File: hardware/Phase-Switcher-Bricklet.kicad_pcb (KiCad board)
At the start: 2 copper layers, 70 x 46.4 mm, 43 parts, among them CN1 HC-GH-7PWTKK, P10 WJ124-3.81-4P, P20 WJ124-3.81-4P, P40 WJ124-3.81-2P, U1 XMC1302-Q024X0032-AB, U10 AQH2223, U11 6N139M, U20 AQH2223, U21 6N139M, U30 AQH2223, U40 AQY282SX

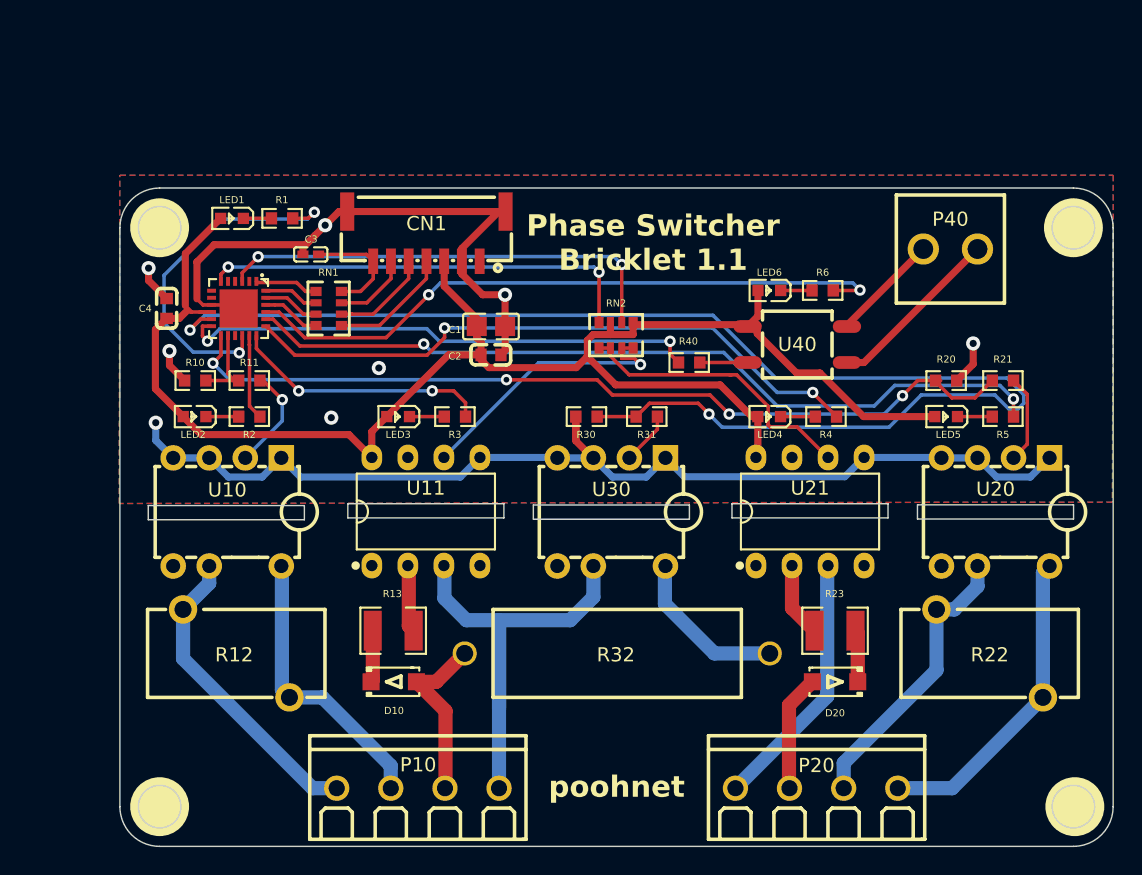
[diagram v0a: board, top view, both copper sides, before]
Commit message: Phase-Switcher-Bricklet: Rev. 1.2
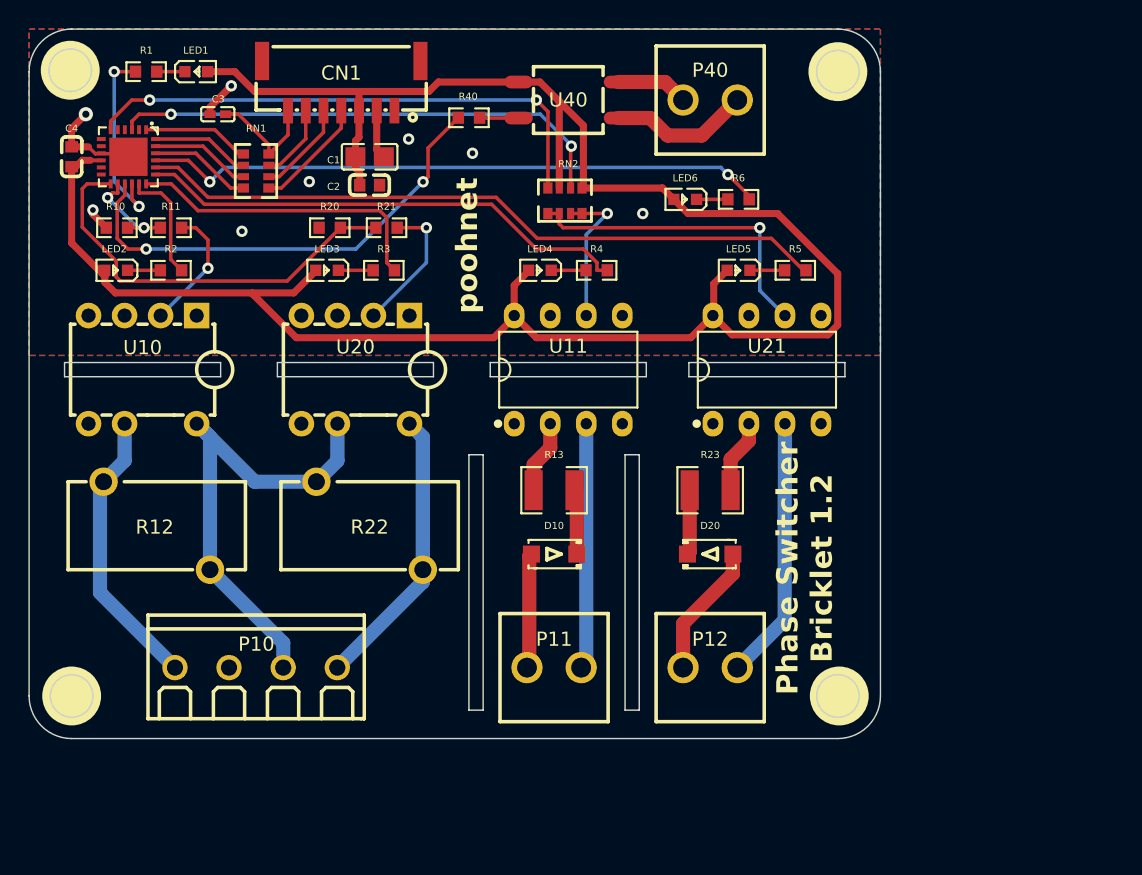
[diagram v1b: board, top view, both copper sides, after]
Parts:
- removed P20: WJ124-3.81-4P, easyeda2kicad:CONN-TH_4P-P3.81_KF124-3.81-4P
- removed R30: 1K, easyeda2kicad:R0603
- removed R31: 150, easyeda2kicad:R0603
- removed R32: RSF5SSJR-73-4K7, easyeda2kicad:RES-TH_BD6.5-L17.5-P21.50-D0.6
- removed U30: AQH2223, easyeda2kicad:DIP-8_7P-L9.7-W6.4-P2.54-LS7.6-BL-PE7
- added P11: WJ124-3.81-2P, easyeda2kicad:CONN-TH_2P-P3.81_KF124-3.81-2P, F.Cu at (87.0, 85.0)
- added P12: WJ124-3.81-2P, easyeda2kicad:CONN-TH_2P-P3.81_KF124-3.81-2P, F.Cu at (98.0, 85.0)
- moved U20 46.2 mm to (73.0, 64.0)
- moved R20 44.8 mm to (71.2, 54.0), turned to 180 degrees
- moved R21 44.8 mm to (75.2, 54.0)
- moved R22 44.6 mm to (74.0, 75.0)
- moved U40 23.6 mm to (88.0, 45.0)
- moved R40 23.2 mm to (81.0, 46.2)
- moved P40 19.9 mm to (98.0, 45.0)
- moved LED4 19.2 mm to (86.0, 57.0)
- moved R4 19.2 mm to (90.0, 57.0)
- moved LED5 17.9 mm to (100.0, 57.0)
- moved R5 17.9 mm to (104.0, 57.0)
- moved R13 15.1 mm to (87.0, 72.5), turned to 0 degrees
- moved C1 14.7 mm to (74.0, 49.0)
- moved C2 14.7 mm to (74.0, 51.0)
- moved D10 14.4 mm to (87.0, 77.0), turned to 180 degrees
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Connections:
- net AC1-1 renamed Net-(U11-VO)
- net AC2-1 renamed Net-(U21-VO)
- P10 pad 1: Net-(U11-VF-) -> Net-(P10-Pad1)
- P10 pad 2: Net-(D10-A) -> Net-(P10-Pad2)
- P10 pad 3: Net-(P10-Pad3) -> unconnected-(P10-Pad3)
- R12 pad 2: Net-(P10-Pad3) -> Net-(P10-Pad2)
- R22 pad 1: Net-(P20-Pad2) -> Net-(P10-Pad2)
- R22 pad 2: Net-(P20-Pad1) -> Net-(P10-Pad1)
- U1 pad 11: RCD -> unconnected-(U1-P1.3-Pad11)
- U1 pad 12: CP -> unconnected-(U1-P1.2-Pad12)
- U1 pad 15: unconnected-(U1-P0.0-Pad15) -> CP
- U10 pad 8: Net-(P10-Pad3) -> Net-(P10-Pad2)
- U20 pad 6: Net-(P20-Pad2) -> Net-(P10-Pad2)
- U20 pad 8: Net-(P20-Pad1) -> Net-(P10-Pad1)
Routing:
- net GND: track 128.8 -> 15.0 mm
- net RCD: track 96.7 -> 0.00 mm, vias 2 -> 0
- net 3V3: track 112.2 -> 150.6 mm
- net Net-(P10-Pad2): track 0.00 -> 34.6 mm
- net Relay2: track 61.0 -> 29.3 mm, vias 4 -> 0
- net Net-(U11-VF-): track 40.0 -> 17.3 mm
- net Net-(P20-Pad1): track 22.3 -> 0.00 mm
- net Net-(P20-Pad2): track 20.8 -> 0.00 mm
- net Net-(P10-Pad3): track 20.3 -> 0.00 mm
- net Net-(P10-Pad1): track 0.00 -> 20.1 mm
- net Net-(R32-Pad1): track 11.5 -> 0.00 mm
- net LED1: track 25.0 -> 13.5 mm
- net LED4: track 44.9 -> 35.0 mm, vias 2 -> 0
- net Net-(U11-VO): track 19.7 -> 10.4 mm
- net LED5: track 57.6 -> 48.8 mm, vias 2 -> 0
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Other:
- board size 70 x 46.4 mm -> 60 x 50 mm
- board text added: "Phase Switcher Bricklet 1.2"
- board text removed: "Phase Switcher Bricklet 1.1"
